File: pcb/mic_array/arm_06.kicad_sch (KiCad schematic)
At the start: 16 parts, among them U49 IM72D128V01XTMA1, U50 IM72D128V01XTMA1, U51 IM72D128V01XTMA1, U52 IM72D128V01XTMA1, U53 IM72D128V01XTMA1, U54 IM72D128V01XTMA1, U55 IM72D128V01XTMA1, U56 IM72D128V01XTMA1

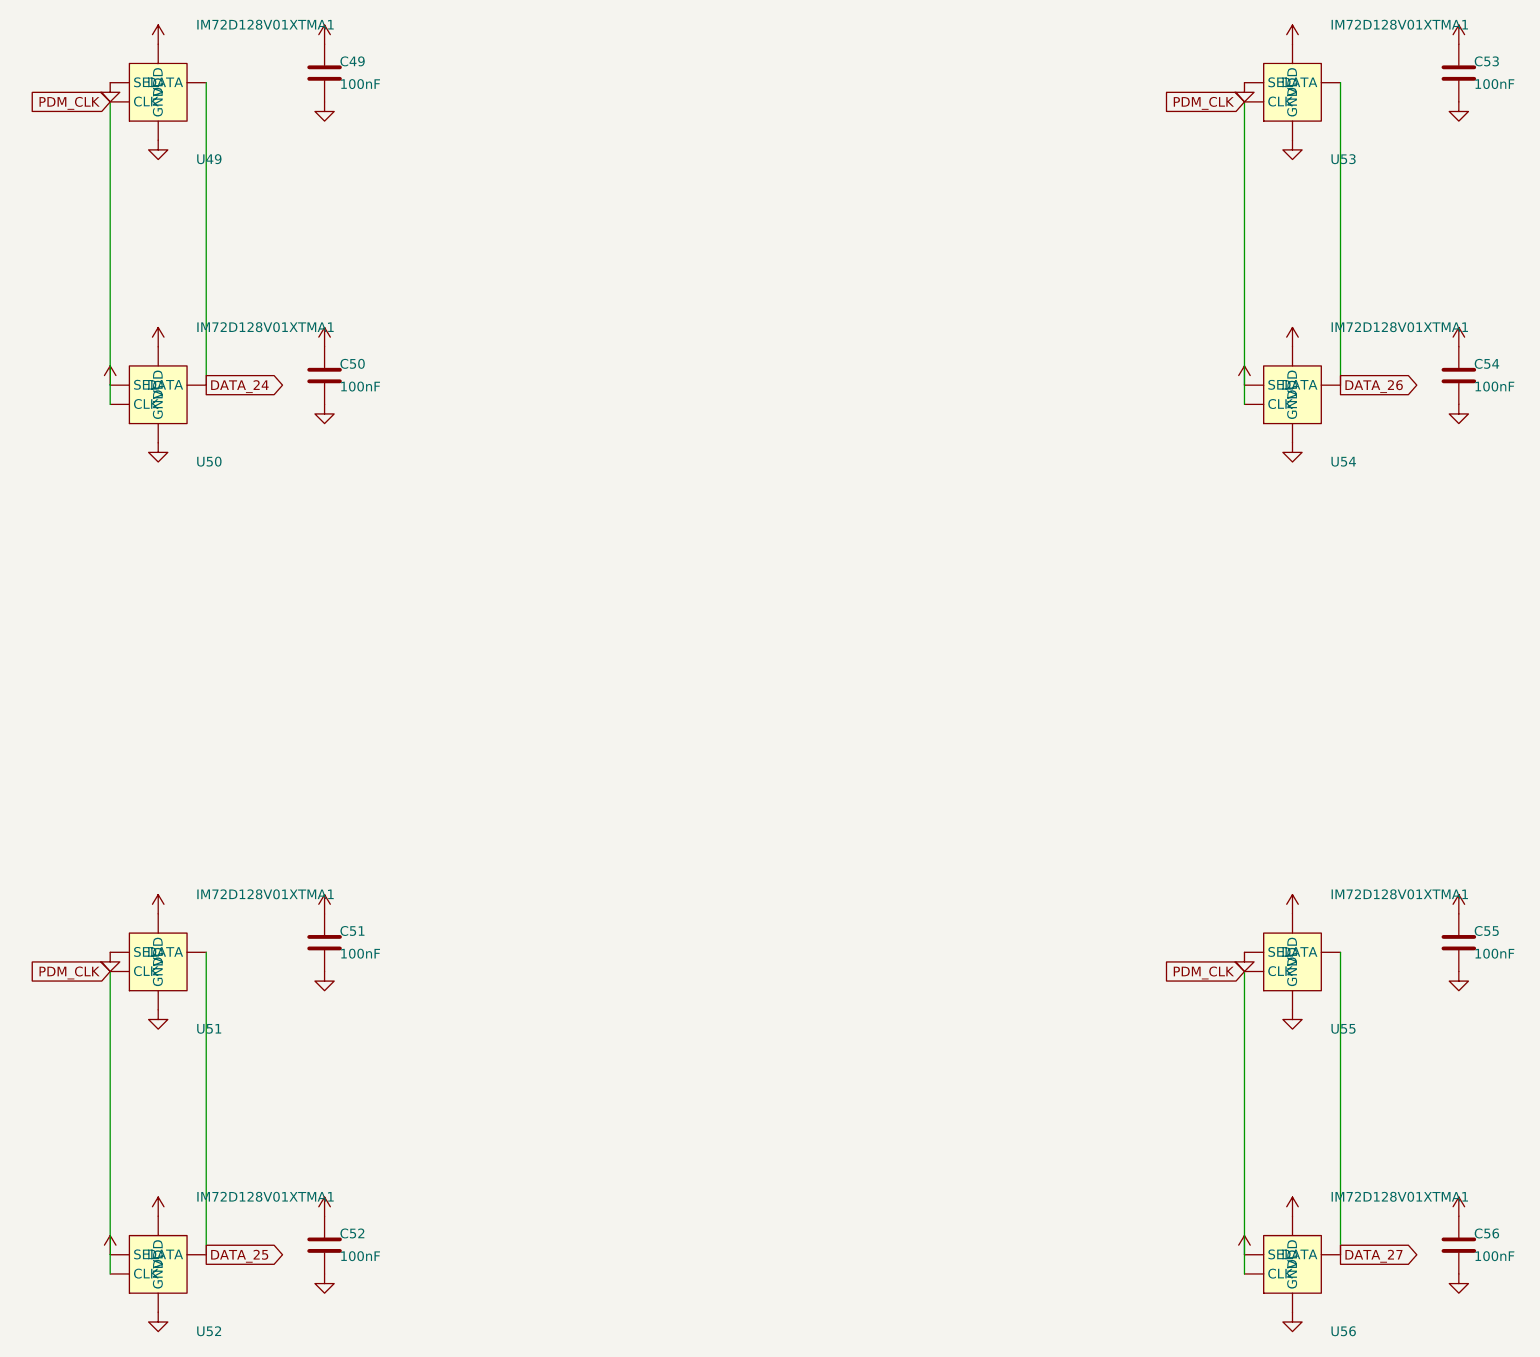
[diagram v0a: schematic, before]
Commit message: Updated.
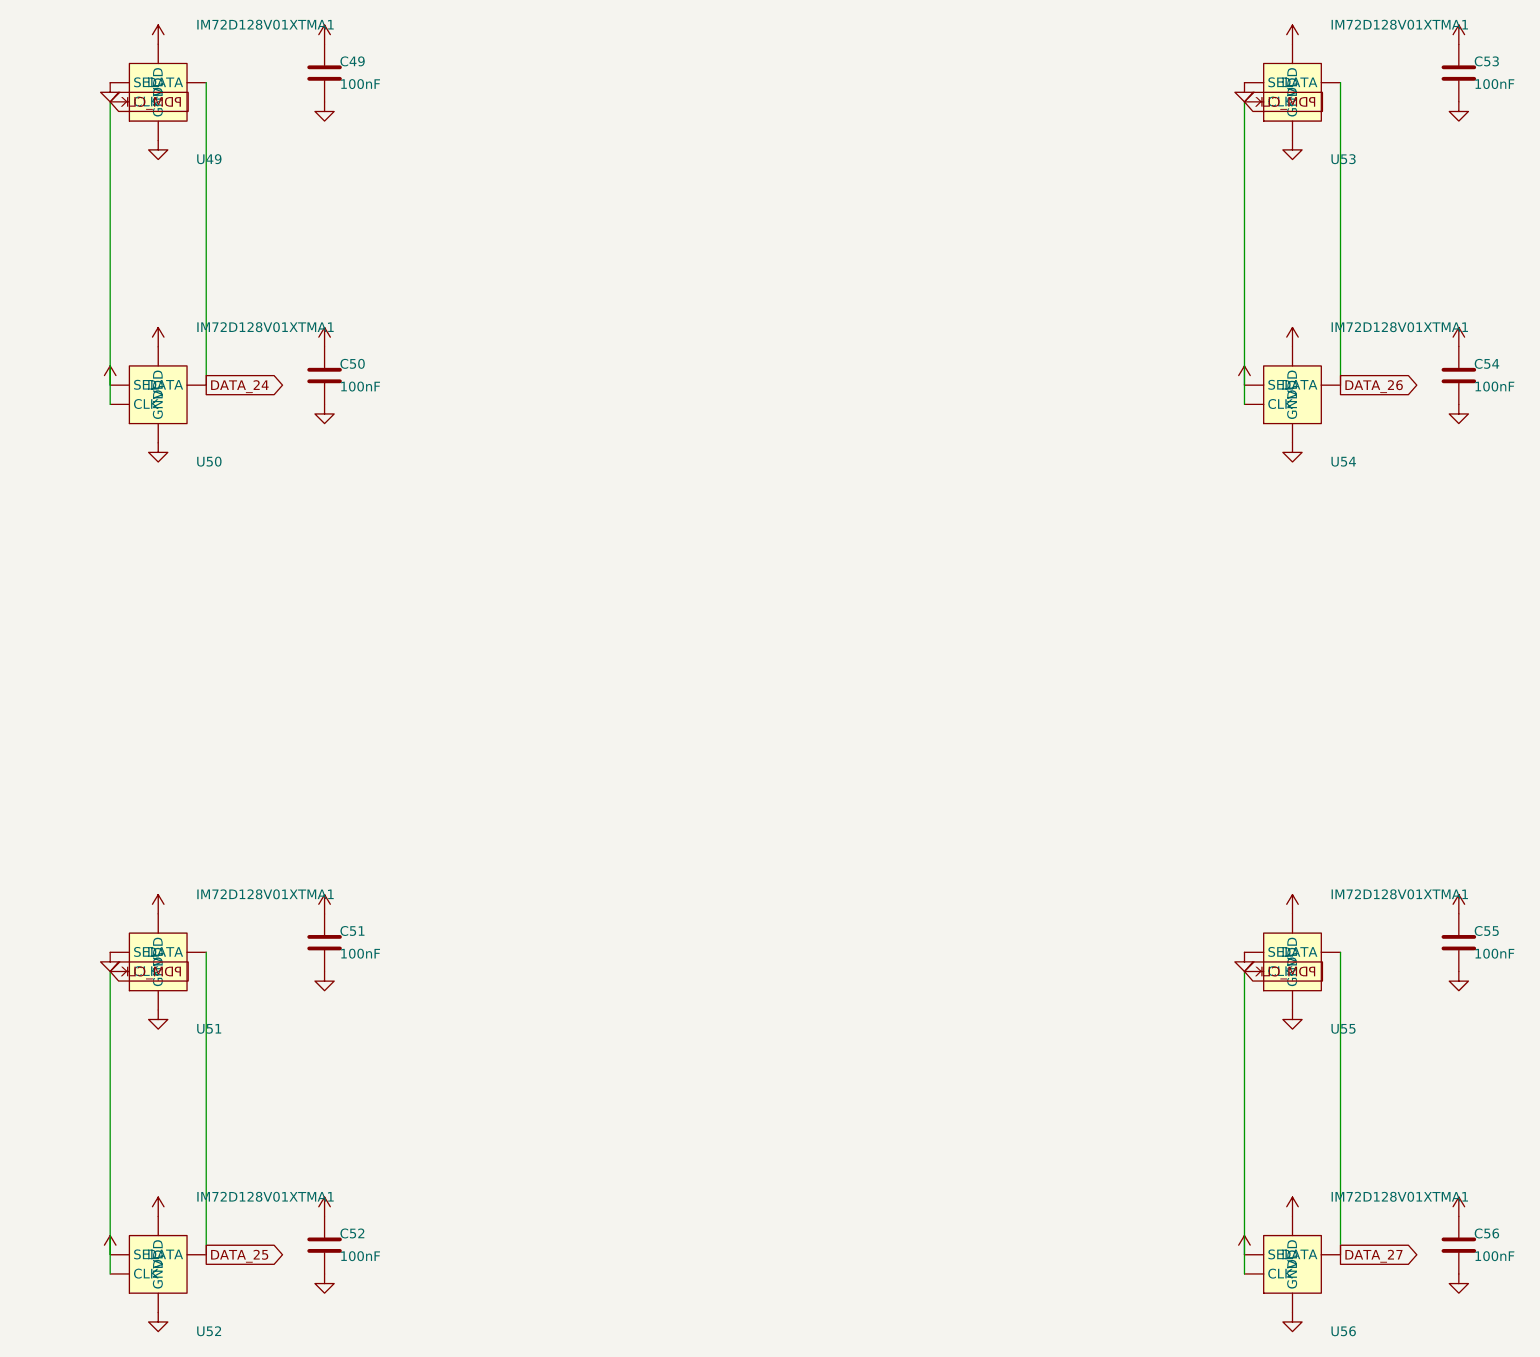
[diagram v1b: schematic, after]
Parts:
- C49, C50, C51, C52, C53, C54, C55, C56: footprint Capacitor_SMD:C_0402_1005Metric -> (none)
- U49, U50, U51, U52, U53, U54, U55, U56: footprint Sensor_Audio:Infineon_PG-LLGA-5-2 -> (none)
